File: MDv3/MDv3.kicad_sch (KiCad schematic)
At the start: 41 parts, among them J1 Conn_01x04_Pin, J3 XT60-M, J4 XT60-M

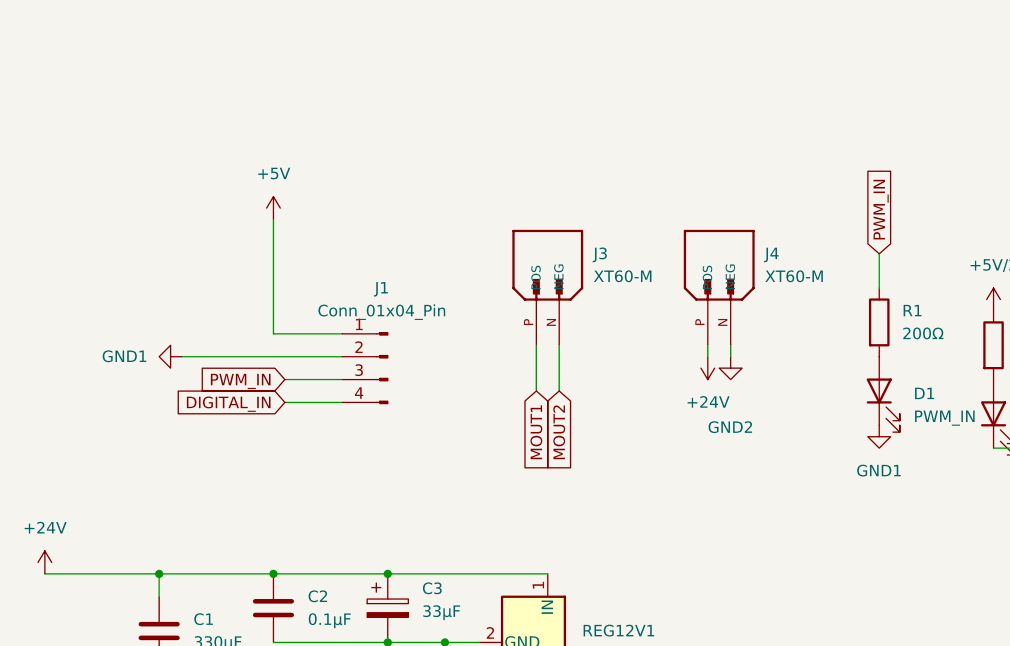
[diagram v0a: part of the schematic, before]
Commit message: やりなおし
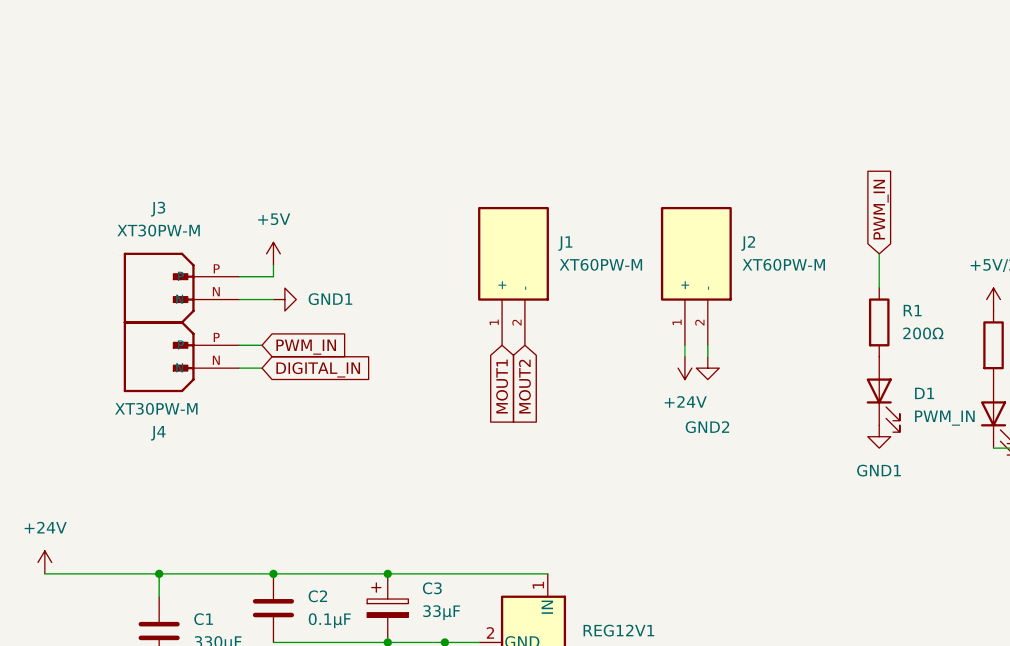
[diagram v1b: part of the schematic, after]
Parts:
- removed J1: Conn_01x04_Pin, Connector_PinHeader_2.54mm:PinHeader_1x04_P2.54mm_Vertical, symbol Connector:Conn_01x04_Pin
- removed J3, J4: XT60-M, XT60-M:AMASS_XT60PW-M, symbol XT60-M:XT60-M
- added J1, J2: XT60PW-M, XT60-M:AMASS_XT60PW-M, symbol XT60PW-M:XT60PW-M
- added J3, J4: XT30PW-M, XT60-M:AMASS_XT30PW-M, symbol XT30UPB-M:XT30PW-M
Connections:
- net +24V: now also J2.1 (+)
- net +5V: now also J3.P
- net DIGITAL_IN: now also J4.N
- net GND1: now also J3.N
- net GND2: now also J2.2 (-)
- net MOUT1: now also J1.1 (+)
- net MOUT2: now also J1.2 (-)
- net PWM_IN: now also J4.P
